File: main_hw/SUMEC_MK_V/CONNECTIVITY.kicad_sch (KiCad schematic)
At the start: 20 parts, among them J4 USB_TypeC, U5 USBLC6-2SC6

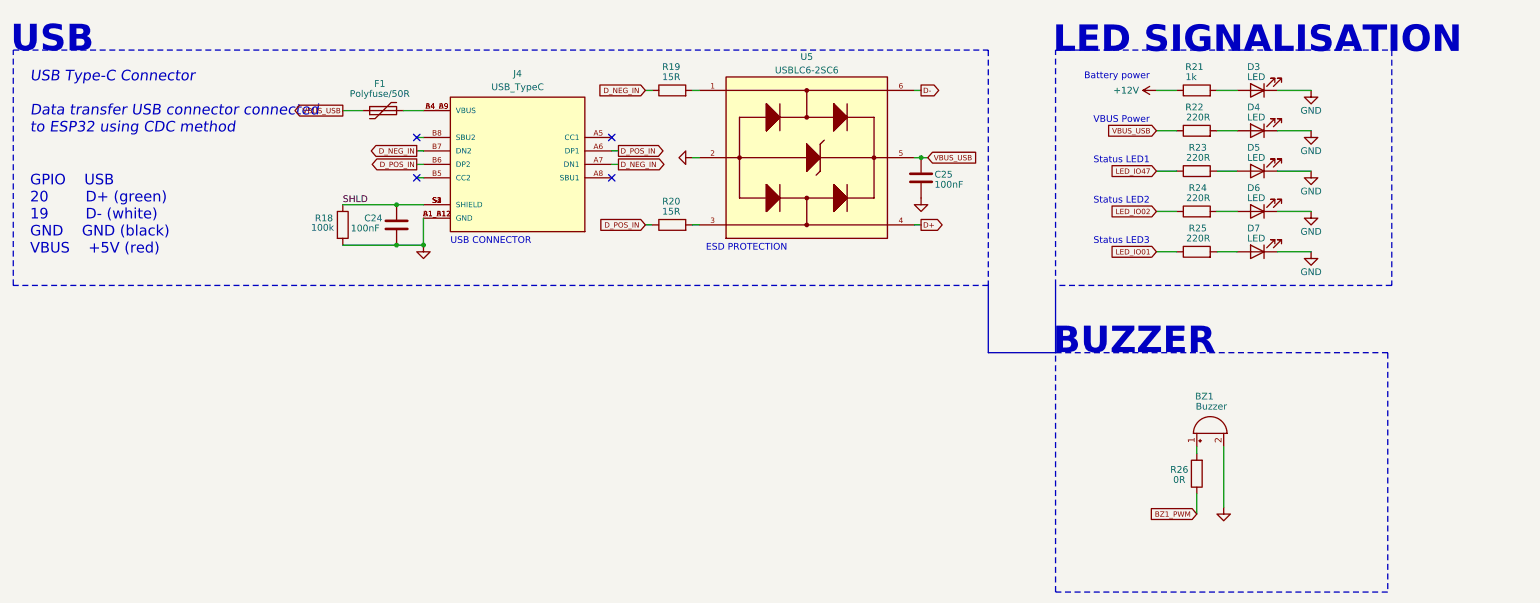
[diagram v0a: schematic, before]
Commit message: new qre board
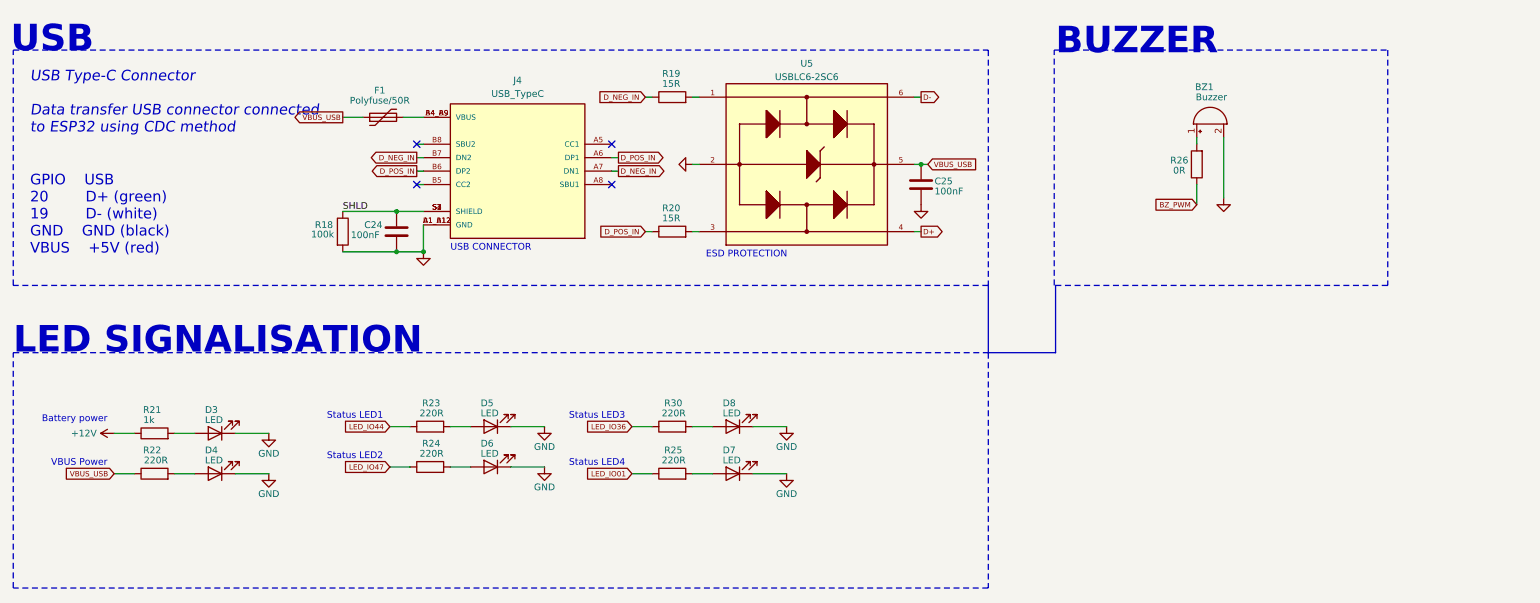
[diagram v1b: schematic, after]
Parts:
- added D8: LED, LED_SMD:LED_0805_2012Metric_Pad1.15x1.40mm_HandSolder, symbol Device:LED
- added R30: 220R, Resistor_SMD:R_0805_2012Metric_Pad1.20x1.40mm_HandSolder, symbol Device:R
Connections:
- net LED_IO02 is gone; now on net LED_IO47: R24.1
- net GND: now also D8.1 (K)
- net LED_IO47: no longer R23.1
- net BZ1_PWM renamed BZ_PWM
- new net: D8.2 (A), R30.2
- new net LED_IO36: R30.1
- new net LED_IO44: R23.1
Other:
- note added: "Status LED4"
- moved on the sheet: BZ1, C24, C25, D3, D4, D5, D6, D7, F1, J4, R18, R19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
